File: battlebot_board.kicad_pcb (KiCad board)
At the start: 4 copper layers, 60 x 45 mm, 43 parts, among them J1 Conn_01x02_Pin, J2 Conn_01x04_Pin, J3 JST_SMD_1.0mm_Vertical, J4 Conn_01x02, J5 JST_02, J6 JST_02, Q1 AO3400A, Q2 AO3400A, SW1 Switch_Tactile_CnK, U1 AP63203WU, U2 LPC824M201JHI33, U3 TMP102, U4 LSM6DSOX, U5 W25Q128JVP

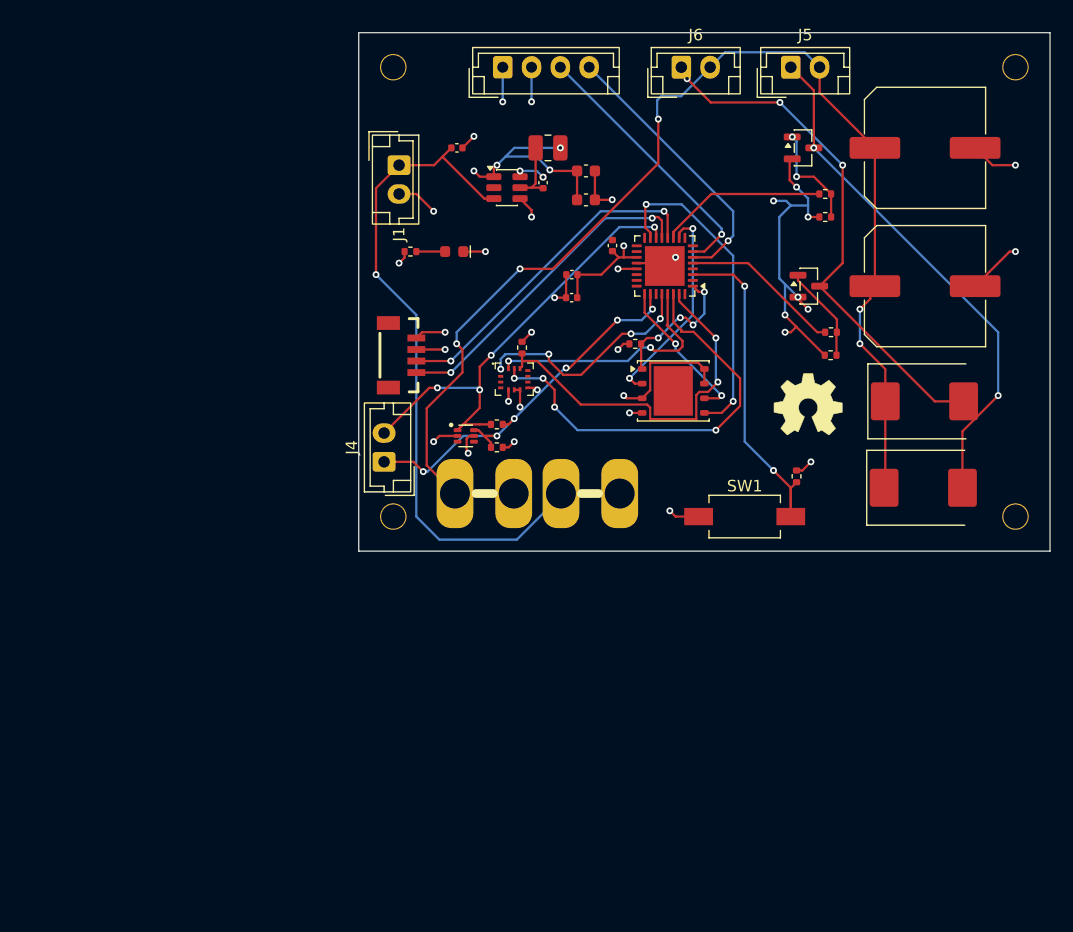
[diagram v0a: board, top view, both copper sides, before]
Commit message: logos and housekeeping
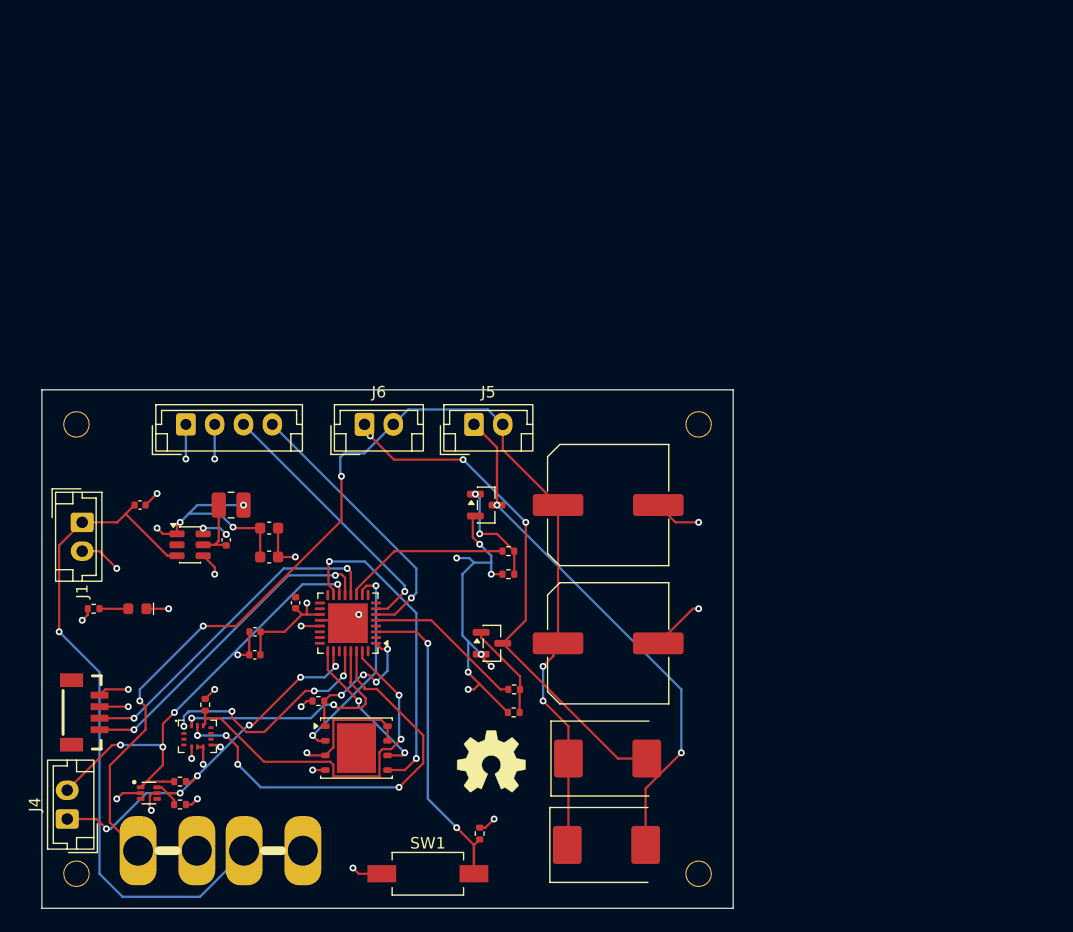
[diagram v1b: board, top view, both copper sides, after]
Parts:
- added G***: LOGO, LOGO, B.Cu at (160.5, 112.0)
- moved C2 41.4 mm to (127.0, 91.0)
- moved R10 41.4 mm to (123.0, 100.0)
- moved C1 41.4 mm to (137.0, 102.0)
- moved C10 41.4 mm to (167.7, 91.0)
- moved C12 41.4 mm to (167.7, 103.0)
- moved C4 41.4 mm to (138.2, 93.0)
- moved C5 41.4 mm to (138.2, 95.5)
- moved C7 41.4 mm to (140.5, 99.5)
- moved C8 41.4 mm to (137.0, 104.0)
- moved D3 41.4 mm to (126.8, 100.0)
- moved D4 41.4 mm to (167.6, 113.0)
- moved D5 41.4 mm to (167.5, 120.5)
- moved F4 41.4 mm to (134.0, 121.0)
- moved H1 41.4 mm to (121.5, 84.0)
- moved H2 41.4 mm to (175.5, 84.0)
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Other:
- board text added: "SDA SCL"
